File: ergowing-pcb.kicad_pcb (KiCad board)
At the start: 2 copper layers, 150 parts, among them J1 USB_mini_micro_B, K0:0 KEYSW, K0:1 KEYSW, K0:2 KEYSW, K0:3 KEYSW, K0:4 KEYSW, K10:0 KEYSW, K10:1 KEYSW, K10:2 KEYSW, K10:3 KEYSW, K10:4 KEYSW, K11:0 KEYSW, K11:1 KEYSW, K11:2 KEYSW, K11:3 KEYSW, K11:4 KEYSW, K12:0 KEYSW, K12:1 KEYSW, K12:2 KEYSW, K12:3 KEYSW, K12:4 KEYSW, K13:0 KEYSW, K13:1 KEYSW, K13:2 KEYSW, K13:3 KEYSW, K13:4 KEYSW, K1:0 KEYSW, K1:1 KEYSW, K1:2 KEYSW, K1:3 KEYSW, K1:4 KEYSW, K2:0 KEYSW, K2:1 KEYSW, K2:2 KEYSW, K2:3 KEYSW, K2:4 KEYSW, K3:0 KEYSW, K3:1 KEYSW, K3:2 KEYSW, K3:3 KEYSW, K3:4 KEYSW, K4:0 KEYSW, K4:1 KEYSW, K4:2 KEYSW, K4:3 KEYSW, K4:4 KEYSW, K5:0 KEYSW, K5:1 KEYSW, K5:2 KEYSW, K5:3 KEYSW, K5:4 KEYSW, K6:0 KEYSW, K6:1 KEYSW, K6:3 KEYSW, K7:0 KEYSW, K7:1 KEYSW, K7:3 KEYSW, K7:4 KEYSW, K8:0 KEYSW, K8:1 KEYSW, K8:2 KEYSW, K8:3 KEYSW, K8:4 KEYSW, K9:0 KEYSW, K9:1 KEYSW, K9:2 KEYSW, K9:3 KEYSW, K9:4 KEYSW, SW1 SW_PUSH, U1 ATMEGA32U4, X1 XTAL_GND

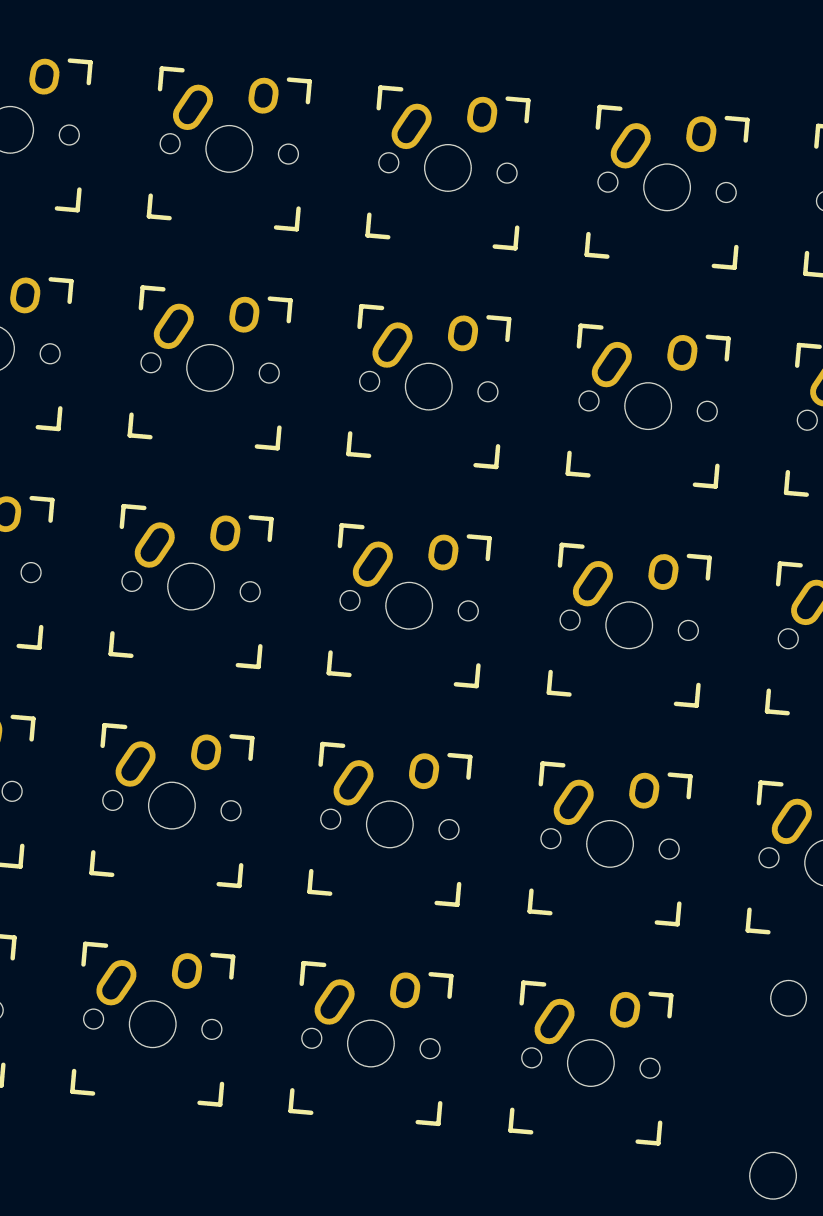
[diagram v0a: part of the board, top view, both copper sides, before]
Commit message: Update #321312
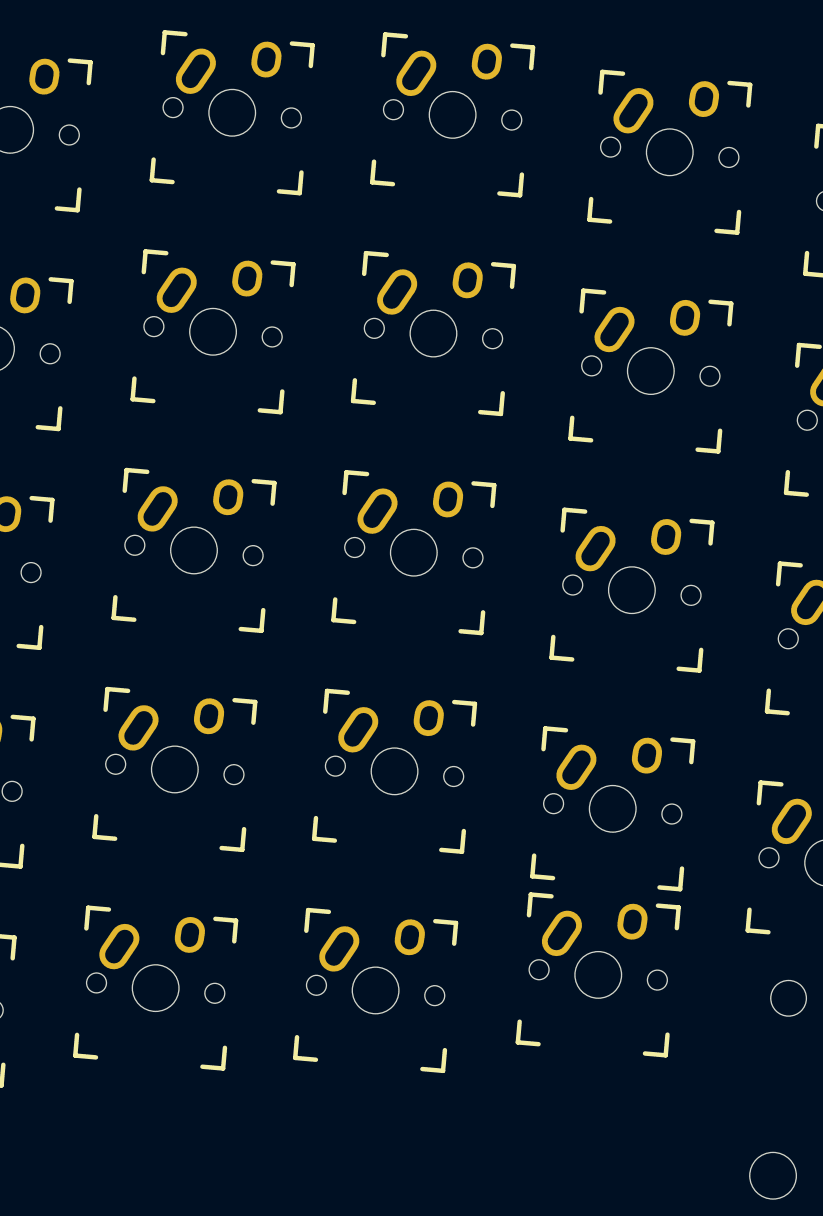
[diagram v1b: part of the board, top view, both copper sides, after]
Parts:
- moved K4:4 7.57 mm to (139.2, 114.1)
- moved K3:4 4.56 mm to (120.2, 115.4)
- moved K3:3 4.56 mm to (121.8, 96.7)
- moved K3:0 4.56 mm to (126.7, 40.5)
- moved K3:1 4.56 mm to (125.1, 59.2)
- moved K3:2 4.56 mm to (123.4, 78.0)
- moved K2:1 3.10 mm to (106.2, 59.0)
- moved K2:3 3.10 mm to (103.0, 96.5)
- moved K2:4 3.10 mm to (101.3, 115.2)
- moved K2:0 3.10 mm to (107.9, 40.3)
- moved K2:2 3.10 mm to (104.6, 77.8)
- moved K4:2 3.01 mm to (142.1, 81.2)
- moved K4:0 3.01 mm to (145.3, 43.7)
- moved K4:1 3.01 mm to (143.7, 62.4)
- moved K4:3 3.01 mm to (140.4, 99.9)
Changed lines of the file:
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@@
     (links 515)
     (no_connects 247)
-    (area 43.748094 28.857392 395.425 379.0775)
+    (area 43.337667 26.864461 395.425 379.0775)
     (thickness 1.6)
     (drawings 0)
@@
   )
   (module keebs:Mx_Alps_100_R-5deg (layer F.Cu)
-    (at 107.63 43.4)
+    (at 107.88 40.31)
     (descr MXALPS)
     (tags MXALPS)
@@
   )
   (module keebs:Mx_Alps_100_R-5deg (layer F.Cu)
-    (at 105.99 62.14)
+    (at 106.24 59.05)
     (descr MXALPS)
     (tags MXALPS)
@@
   )
   (module keebs:Mx_Alps_100_R-5deg (layer F.Cu)
-    (at 104.36 80.85)
+    (at 104.61 77.76)
     (descr MXALPS)
     (tags MXALPS)
@@
   )
   (module keebs:Mx_Alps_100_R-5deg (layer F.Cu)
-    (at 102.72 99.59)
+    (at 102.97 96.5)
     (descr MXALPS)
     (tags MXALPS)
@@
   )
   (module keebs:Mx_Alps_100_R-5deg (layer F.Cu)
-    (at 101.08 118.3)
+    (at 101.33 115.21)
     (descr MXALPS)
     (tags MXALPS)
@@
   )
   (module keebs:Mx_Alps_100_R-5deg (layer F.Cu)
-    (at 126.34 45.03)
+    (at 126.74 40.49)
     (descr MXALPS)
     (tags MXALPS)
@@
   )
   (module keebs:Mx_Alps_100_R-5deg (layer F.Cu)
-    (at 124.7 63.74)
+    (at 125.1 59.2)
     (descr MXALPS)
     (tags MXALPS)
@@
   )
   (module keebs:Mx_Alps_100_R-5deg (layer F.Cu)
-    (at 123.02 82.49)
+    (at 123.42 77.95)
     (descr MXALPS)
     (tags MXALPS)
@@
   )
   (module keebs:Mx_Alps_100_R-5deg (layer F.Cu)
-    (at 121.37 101.2)
+    (at 121.77 96.66)
     (descr MXALPS)
     (tags MXALPS)
@@
   )
   (module keebs:Mx_Alps_100_R-5deg (layer F.Cu)
-    (at 119.75 119.95)
+    (at 120.15 115.41)
     (descr MXALPS)
     (tags MXALPS)
@@
   )
   (module keebs:Mx_Alps_100_R-5deg (layer F.Cu)
-    (at 145.09 46.69)
+    (at 145.32 43.69)
     (descr MXALPS)
     (tags MXALPS)
@@
   )
   (module keebs:Mx_Alps_100_R-5deg (layer F.Cu)
-    (at 143.47 65.41)
+    (at 143.7 62.41)
     (descr MXALPS)
     (tags MXALPS)
@@
   )
   (module keebs:Mx_Alps_100_R-5deg (layer F.Cu)
-    (at 141.85 84.16)
+    (at 142.08 81.16)
     (descr MXALPS)
     (tags MXALPS)
@@
   )
   (module keebs:Mx_Alps_100_R-5deg (layer F.Cu)
-    (at 140.21 102.87)
+    (at 140.44 99.87)
     (descr MXALPS)
     (tags MXALPS)
@@
   )
   (module keebs:Mx_Alps_100_R-5deg (layer F.Cu)
-    (at 138.57 121.62)
+    (at 139.2 114.08)
     (descr MXALPS)
     (tags MXALPS)

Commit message: Revert "Update #321312"
This reverts commit 362bd967889284bfad0d96aa47e5c379ba675c40.
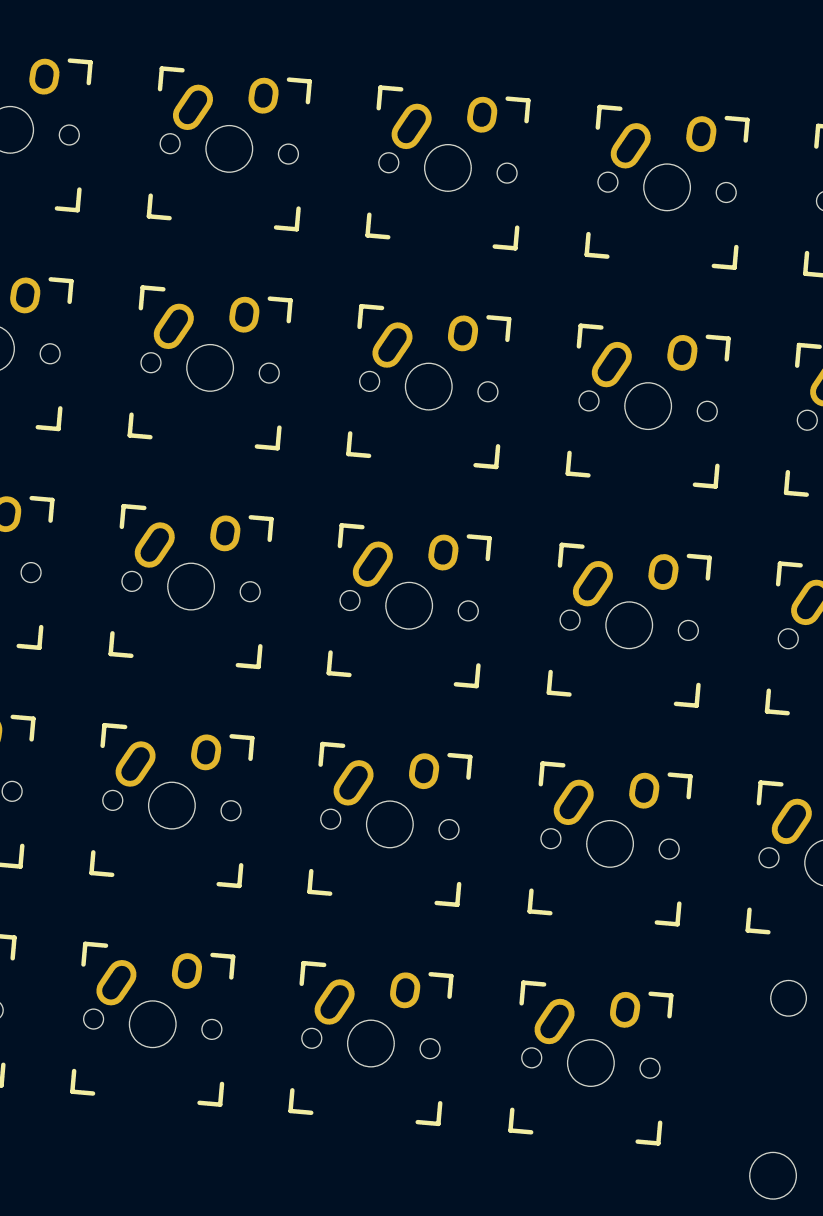
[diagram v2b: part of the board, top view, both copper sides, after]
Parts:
- moved K4:4 7.57 mm to (138.6, 121.6)
- moved K3:4 4.56 mm to (119.8, 120.0)
- moved K3:3 4.56 mm to (121.4, 101.2)
- moved K3:0 4.56 mm to (126.3, 45.0)
- moved K3:1 4.56 mm to (124.7, 63.7)
- moved K3:2 4.56 mm to (123.0, 82.5)
- moved K2:1 3.10 mm to (106.0, 62.1)
- moved K2:3 3.10 mm to (102.7, 99.6)
- moved K2:4 3.10 mm to (101.1, 118.3)
- moved K2:0 3.10 mm to (107.6, 43.4)
- moved K2:2 3.10 mm to (104.4, 80.8)
- moved K4:2 3.01 mm to (141.8, 84.2)
- moved K4:0 3.01 mm to (145.1, 46.7)
- moved K4:1 3.01 mm to (143.5, 65.4)
- moved K4:3 3.01 mm to (140.2, 102.9)
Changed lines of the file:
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@@
     (links 515)
     (no_connects 247)
-    (area 43.337667 26.864461 395.425 379.0775)
+    (area 43.748094 28.857392 395.425 379.0775)
     (thickness 1.6)
     (drawings 0)
@@
   )
   (module keebs:Mx_Alps_100_R-5deg (layer F.Cu)
-    (at 107.88 40.31)
+    (at 107.63 43.4)
     (descr MXALPS)
     (tags MXALPS)
@@
   )
   (module keebs:Mx_Alps_100_R-5deg (layer F.Cu)
-    (at 106.24 59.05)
+    (at 105.99 62.14)
     (descr MXALPS)
     (tags MXALPS)
@@
   )
   (module keebs:Mx_Alps_100_R-5deg (layer F.Cu)
-    (at 104.61 77.76)
+    (at 104.36 80.85)
     (descr MXALPS)
     (tags MXALPS)
@@
   )
   (module keebs:Mx_Alps_100_R-5deg (layer F.Cu)
-    (at 102.97 96.5)
+    (at 102.72 99.59)
     (descr MXALPS)
     (tags MXALPS)
@@
   )
   (module keebs:Mx_Alps_100_R-5deg (layer F.Cu)
-    (at 101.33 115.21)
+    (at 101.08 118.3)
     (descr MXALPS)
     (tags MXALPS)
@@
   )
   (module keebs:Mx_Alps_100_R-5deg (layer F.Cu)
-    (at 126.74 40.49)
+    (at 126.34 45.03)
     (descr MXALPS)
     (tags MXALPS)
@@
   )
   (module keebs:Mx_Alps_100_R-5deg (layer F.Cu)
-    (at 125.1 59.2)
+    (at 124.7 63.74)
     (descr MXALPS)
     (tags MXALPS)
@@
   )
   (module keebs:Mx_Alps_100_R-5deg (layer F.Cu)
-    (at 123.42 77.95)
+    (at 123.02 82.49)
     (descr MXALPS)
     (tags MXALPS)
@@
   )
   (module keebs:Mx_Alps_100_R-5deg (layer F.Cu)
-    (at 121.77 96.66)
+    (at 121.37 101.2)
     (descr MXALPS)
     (tags MXALPS)
@@
   )
   (module keebs:Mx_Alps_100_R-5deg (layer F.Cu)
-    (at 120.15 115.41)
+    (at 119.75 119.95)
     (descr MXALPS)
     (tags MXALPS)
@@
   )
   (module keebs:Mx_Alps_100_R-5deg (layer F.Cu)
-    (at 145.32 43.69)
+    (at 145.09 46.69)
     (descr MXALPS)
     (tags MXALPS)
@@
   )
   (module keebs:Mx_Alps_100_R-5deg (layer F.Cu)
-    (at 143.7 62.41)
+    (at 143.47 65.41)
     (descr MXALPS)
     (tags MXALPS)
@@
   )
   (module keebs:Mx_Alps_100_R-5deg (layer F.Cu)
-    (at 142.08 81.16)
+    (at 141.85 84.16)
     (descr MXALPS)
     (tags MXALPS)
@@
   )
   (module keebs:Mx_Alps_100_R-5deg (layer F.Cu)
-    (at 140.44 99.87)
+    (at 140.21 102.87)
     (descr MXALPS)
     (tags MXALPS)
@@
   )
   (module keebs:Mx_Alps_100_R-5deg (layer F.Cu)
-    (at 139.2 114.08)
+    (at 138.57 121.62)
     (descr MXALPS)
     (tags MXALPS)
